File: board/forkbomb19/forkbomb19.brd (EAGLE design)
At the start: 100 x 100 mm, 30 parts, among them U1 ESP-WROOM-03

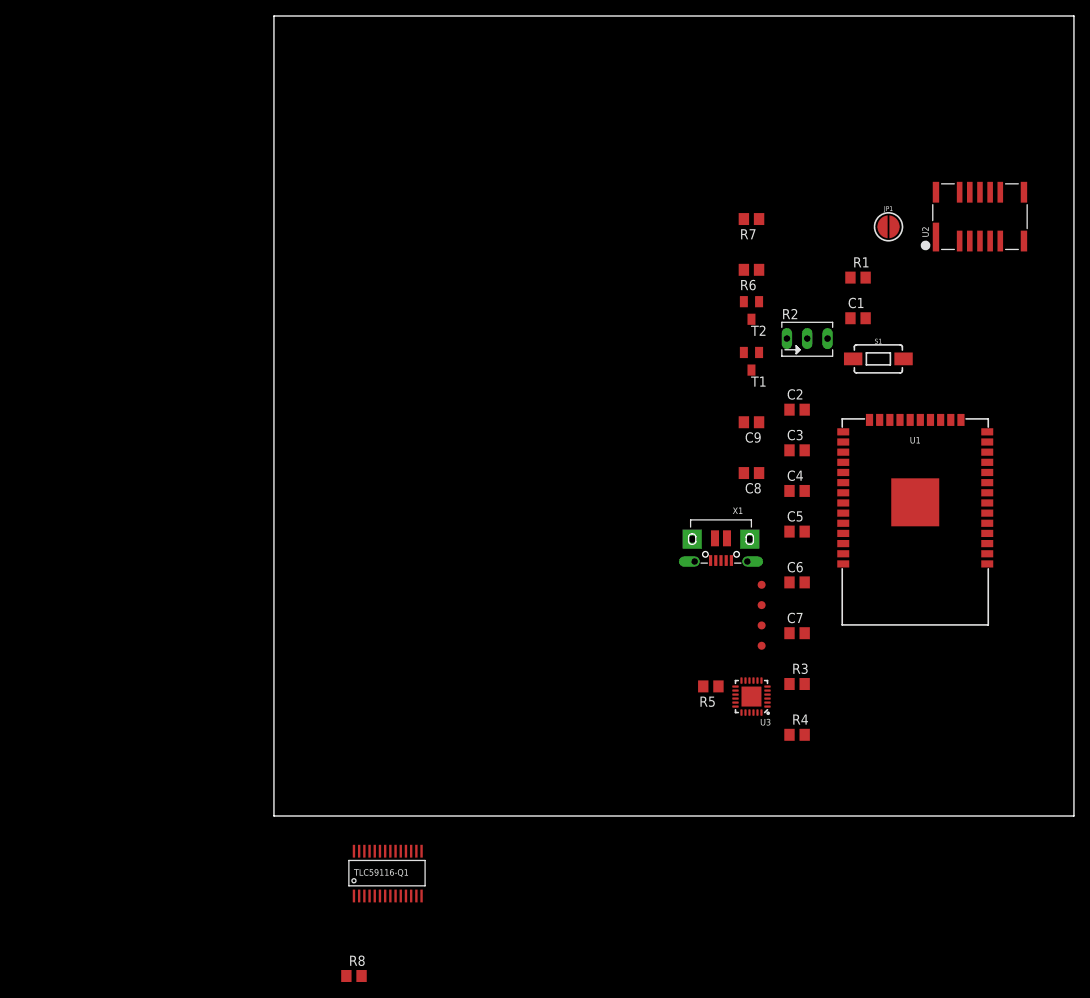
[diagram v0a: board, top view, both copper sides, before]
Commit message: drew the tv and started placing stuff
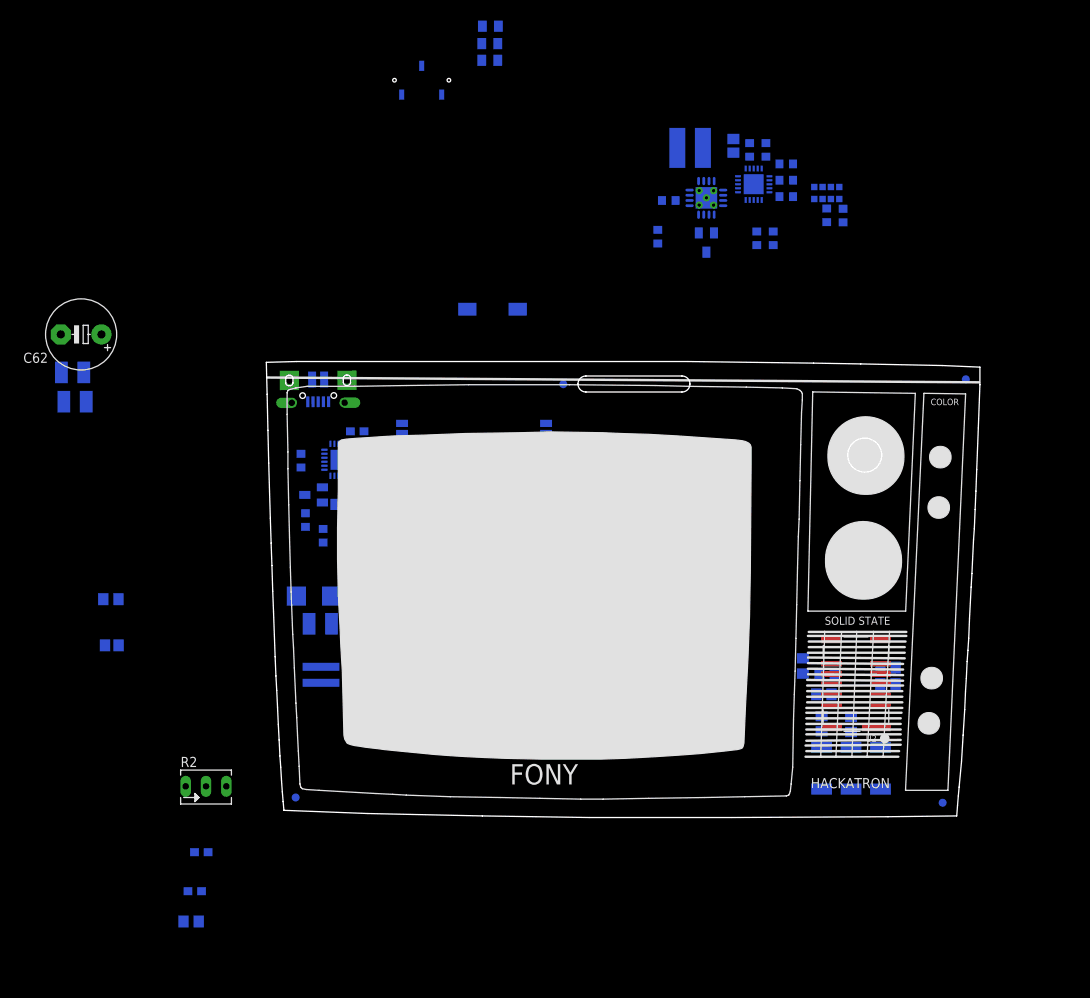
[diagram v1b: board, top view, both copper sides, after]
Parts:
- removed U$1: TLC59116-Q1, forkbomb19:TSSOP28
- added C10, C13, C14: 10uF, resistor:C1210
- added C11: 2.2uF, adafruit:C0805
- added C12: 0.1uF, adafruit:C0805
- added C62: 1F, resistor:E5-8,5
- added CHRG/LBO: ORANGE, piboy_new:ADAFRUIT_CHIPLED_0603
- added CN1: LIPO, adafruit:JST-PH-2-SMT-RA
- added D1: MBRS130LT3, diode:SMB
- added DONE: GREEN, piboy_new:ADAFRUIT_CHIPLED_0603
- added L1: 6.8uH, microbuilder:INDUCTOR_5X5MM_TDK_VLC5045
- added LBO: RED, piboy_new:ADAFRUIT_CHIPLED_0603
- added LOGO_B, LOGO_G, LOGO_R: (no value), forkbomb19:PLCC2_LED
- added ON: BLUE, piboy_new:ADAFRUIT_CHIPLED_0603
- added R10: 1.12M, resistor:R0603
- added R11: 200K, resistor:R0603
- added R12: 340K, adafruit:R0805
- added R13: 200K, adafruit:R0805
- added R14: 1.87M, adafruit:R0805
- added R15: 270K, resistor:R0603
- added R16, R21: 100K, resistor:R0603
- added R17, R18, R20, R9: 1K, resistor:R0603
- added R19: 1.0K, resistor:R0603
- added R22: 68, resistor:R0805
- added T3: MMUN2133LT1G, piboy_new:TRANSISTOR_SC59-BEC
- added THERM: 15K, resistor:R0603
- added U$17: CL-SB-12A-02T, defcon:CL-SB-12A-02T
- added U4: TPS61090RSAR, microbuilder:PVQFN-16
- added U5: MCP73871, microbuilder:QFN20_4MM
- C1: value (none) -> 100nF; device resistor:C0805 -> resistor:C0603
- C4, C9: device resistor:C0805 -> resistor:C0603
- R1, R6, R7: device resistor:R0805 -> resistor:R0603
- R8: value ILED -> 68
- moved R2 93.7 mm to (-8.49, 3.71)
- moved C9 91.0 mm to (-9.90, -9.40), flipped to the bottom, turned to 0 degrees
- moved C8 89.7 mm to (-10.4, -13.2), flipped to the bottom, turned to 0 degrees
- moved C4 87.1 mm to (-9.08, -4.52), flipped to the bottom
- moved C5 86.2 mm to (-20.4, 27.1), flipped to the bottom
- moved R1 75.4 mm to (3.94, 37.0), flipped to the bottom, turned to 270 degrees
- moved R8 69.6 mm to (72.1, 11.5), flipped to the bottom, turned to 270 degrees
- moved C1 64.2 mm to (10.4, 48.1), flipped to the bottom, turned to 180 degrees
- moved R7 63.9 mm to (3.37, 44.4), flipped to the bottom, turned to 90 degrees
- moved R6 63.0 mm to (6.15, 35.0), flipped to the bottom, turned to 270 degrees
- moved FID1 61.3 mm to (2.71, 2.32), flipped to the bottom
- moved U2 60.5 mm to (72.8, 16.5), turned to 90 degrees
- moved T2 59.4 mm to (4.96, 40.1), flipped to the bottom, turned to 270 degrees
- moved U3 59.3 mm to (8.31, 44.5), flipped to the bottom, turned to 270 degrees
- moved C2 57.0 mm to (13.5, 27.4), flipped to the bottom
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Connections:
- removed net RDY_2_SEND: U3.19
- new net BOOST_ENABLE: R13.2, U$17.P$2, U4.11
- new net LBO: T3.B, U4.12
- new net N$16: L1.P$2, U4.3, U4.4
- new net N$17: R12.2, R14.1, U4.9
- new net N$18: LBO.A, R20.1
- new net N$19: R10.1, R11.2, U4.14
- new net N$20: R20.2, T3.C
- new net N$21: ON.A, R9.2
- new net N$22: R15.1, R16.1, U5.P$2
- new net N$23: R18.1, U5.P$7
- new net N$24: R17.1, U5.P$8
- new net N$25: R19.2, U5.P$13
- new net N$26: THERM.2, U5.P$5
- new net N$27: DONE.C, R18.2
- new net N$28: CHRG/LBO.C, R17.2
- new net N$29: R21.2, U5.P$12
- new net N$30: CN1.1, D1.A
- new net N$31: LOGO_G.1, R8.2
- new net VBAT: C10.1, C12.1, L1.P$1, R13.1, R14.2, T3.E, U4.8, U5.P$1, U5.P$20
- new net VBUS: CHRG/LBO.A, DONE.A, R15.2, U5.P$17, U5.P$18, U5.P$19, U5.P$3, U5.P$4, U5.P$9
- new net VLIPO: C14.1, D1.C, U5.P$14, U5.P$15, U5.P$16
- net +3V3: now also C11.1, C13.1, C62.+, LOGO_B.1, R10.2, R22.1, R8.1, R9.1, U4.1, U4.15, U4.16; no longer U$1.P$28
- net EN: no longer U$1.P$25
- net GND: now also C10.2, C11.2, C12.2, C13.2, C14.2, C62.-, CN1.2, LBO.C, LOGO_B.2, LOGO_G.2, LOGO_R.2, ON.C, R11.1, R12.1, R16.2, R19.1, R21.1, THERM.1, U$17.P$3, U4.10, U4.13, U4.5, U4.6, U4.7, U4.P$18, U4.P$19, U4.P$20, U4.P$21, U4.P$22, U4.THERMAL, U5.P$10, U5.P$11, U5.P$21; no longer R8.1, U$1.P$10, U$1.P$19, U$1.P$2, U$1.P$24, U$1.P$3, U$1.P$4, U$1.P$5
- net I2C_SCL: no longer U$1.P$26
- net I2C_SDA: no longer U$1.P$27
- net N$12: now also LOGO_R.1, R22.2; no longer R8.2, U$1.P$1
- net RDY_2_SND: now also U3.19
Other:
- board size 100 x 100 mm -> 89.2 x 57 mm
- board text added: "COLOR"
- board text added: "FONY"
- board text added: "HACKATRON"
- board text added: "SOLID STATE"
